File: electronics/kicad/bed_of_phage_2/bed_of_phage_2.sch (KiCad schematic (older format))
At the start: 14 parts, among them J1 CONN_03, J2 CONN_03, P1 CONN_8, U1 LM358N, U2 LM358N

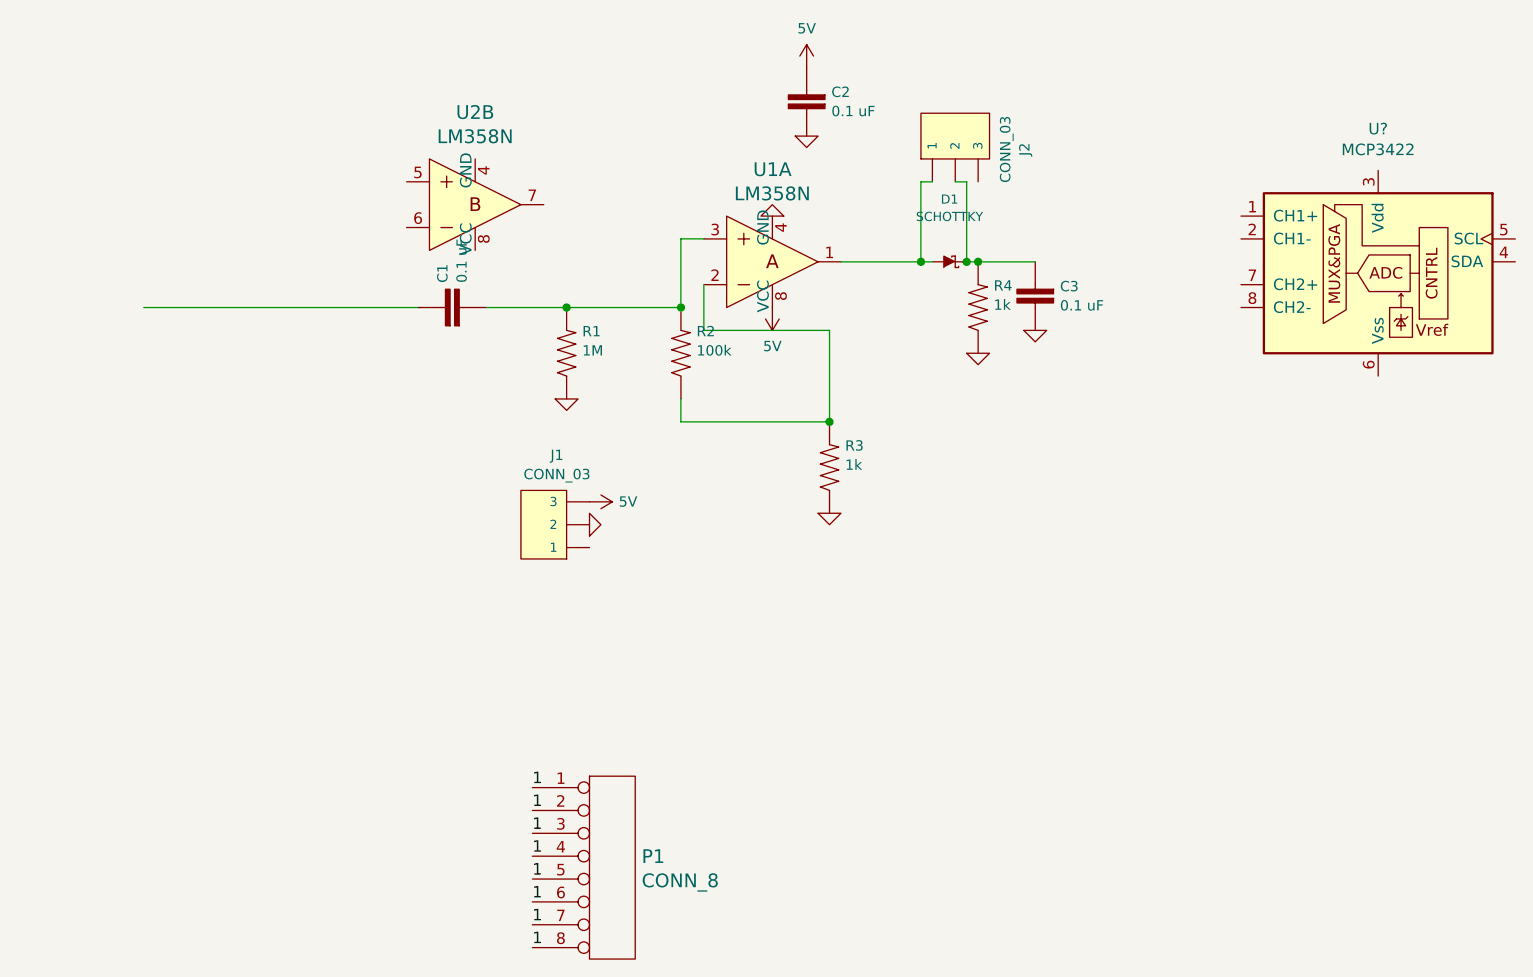
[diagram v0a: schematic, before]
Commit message: nope, I didn't screw that up.
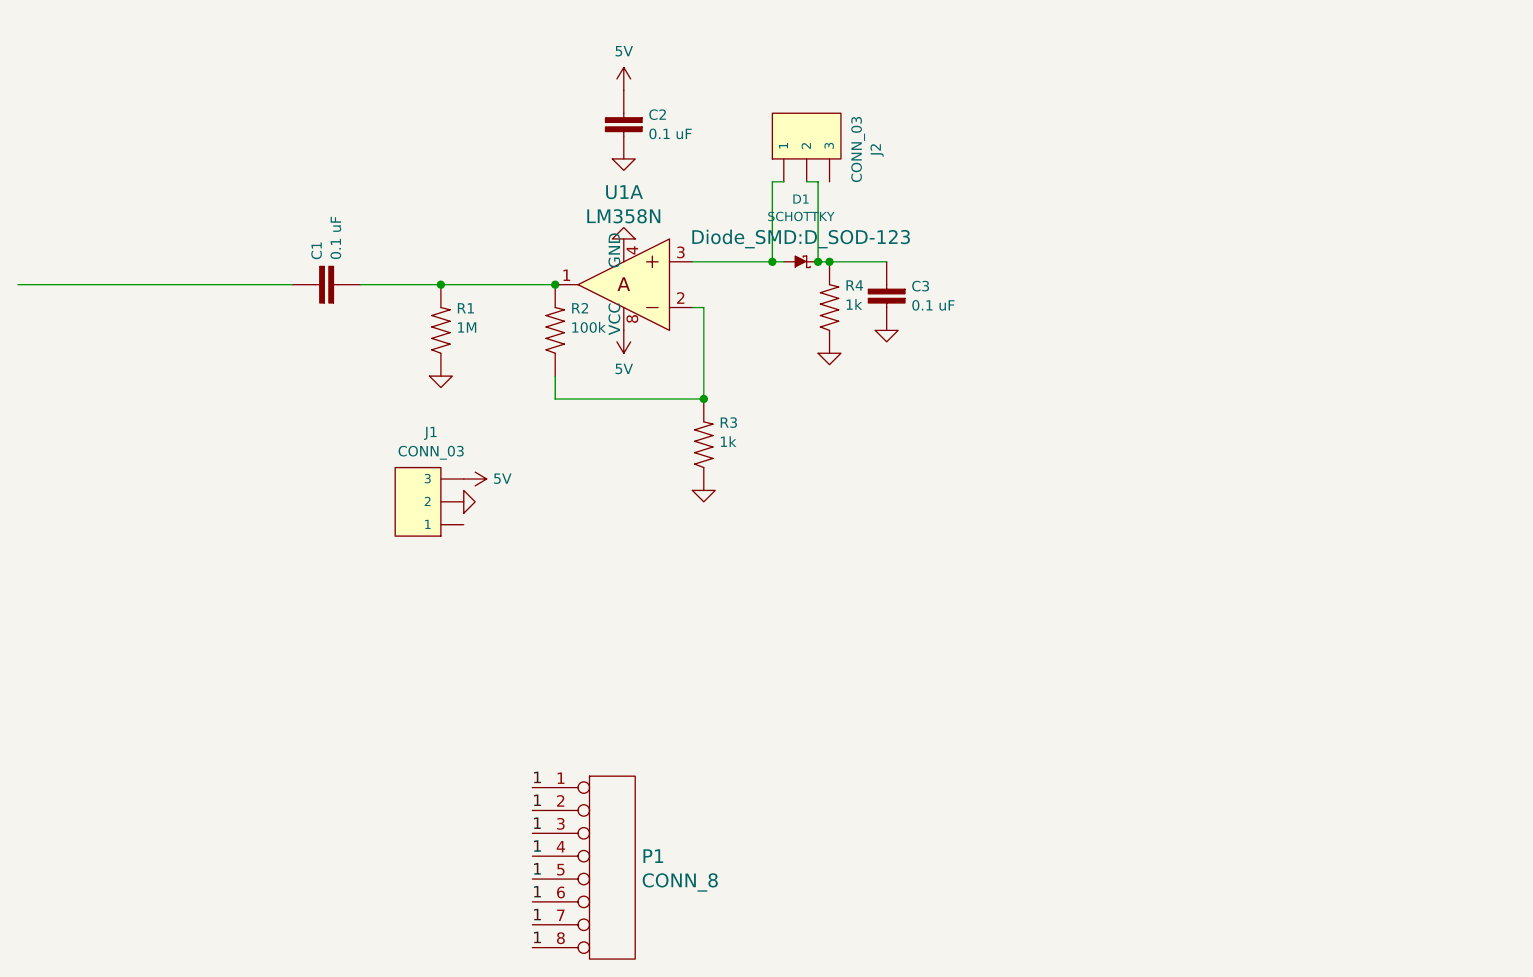
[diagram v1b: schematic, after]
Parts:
- removed U2: LM358N, digikey-footprints:DIP-8_W7.62mm, symbol dk_Linear-Amplifiers-Instrumentation-OP-Amps-Buffer-Amps:LM358N
- removed U?: MCP3422, symbol Analog_ADC:MCP3422
- D1: footprint (none) -> Diode_SMD:D_SOD-123
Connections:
- wire segments 18 -> 15
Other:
- moved on the sheet: C1, C2, C3, D1, J1, J2, R1, R2, R3, R4, U1A
